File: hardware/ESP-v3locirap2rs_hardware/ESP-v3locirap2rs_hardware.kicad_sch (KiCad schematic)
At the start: 2 parts, among them U1 ESP32-DEVKITC-32D

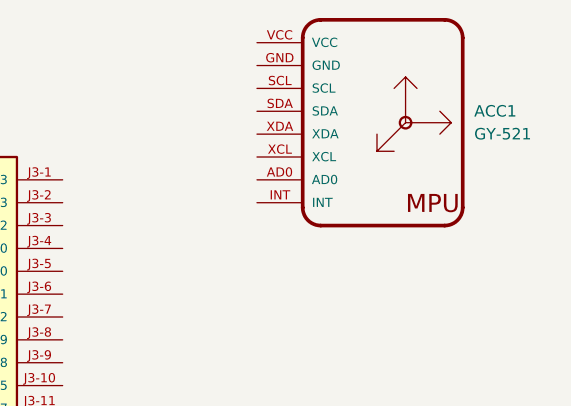
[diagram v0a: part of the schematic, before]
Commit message: updates
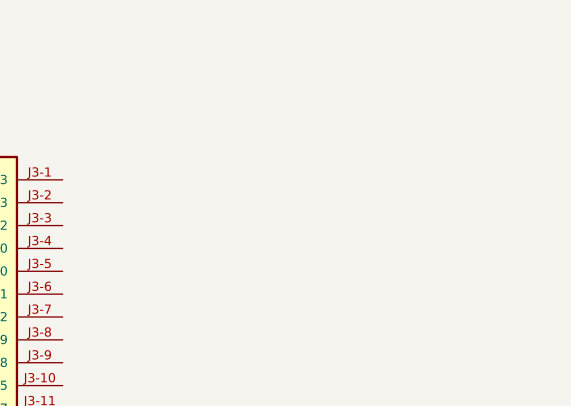
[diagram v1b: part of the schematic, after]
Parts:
- removed ACC1: GY-521, ESP-v3locirap2rs_footprints:GY-521, symbol GY-521:GY-521
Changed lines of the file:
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@@
 	(paper "A4")
-	(symbol
-		(lib_id "GY-521:GY-521")
-		(at 199.39 74.93 0)
-		(unit 1)
-		(exclude_from_sim no)
-		(in_bom yes)
-		(on_board yes)
-		(dnp no)
-		(fields_autoplaced yes)
-		(property "Reference" "ACC1"
-			(at 207.01 73.6599 0)
-			(effects
-				(font
-					(size 1.27 1.27)
-				)
-				(justify left)
-			)
-		)
-		(property "Value" "GY-521"
-			(at 207.01 76.1999 0)
-			(effects
-				(font
-					(size 1.27 1.27)
-				)
-				(justify left)
-			)
-		)
-		(property "Footprint" "ESP-v3locirap2rs_footprints:GY-521"
-			(at 199.39 74.93 0)
-			(effects
-				(font
-					(size 1.27 1.27)
-				)
-				(hide yes)
-			)
-		)
-		(property "Datasheet" ""
-			(at 199.39 74.93 0)
-			(effects
-				(font
-					(size 1.27 1.27)
-				)
-				(hide yes)
-			)
-		)
-		(property "Description" ""
-			(at 199.39 74.93 0)
-			(effects
-				(font
-					(size 1.27 1.27)
-				)
-				(hide yes)
-			)
-		)
-		(property "MF" "GODREAM FORDREAM CO., LIMITED"
-			(at 199.39 74.93 0)
-			(effects
-				(font
-					(size 1.27 1.27)
-				)
-				(justify bottom)
-				(hide yes)
-			)
-		)
-		(property "Description_1" "\n                        \n                            Triple Axis Accelerometer Gyro Breakout\n                        \n"
-			(at 199.39 74.93 0)
-			(effects
-				(font
-					(size 1.27 1.27)
-				)
-				(justify bottom)
-				(hide yes)
-			)
-		)
-		(property "Package" "Package"
-			(at 199.39 74.93 0)
-			(effects
-				(font
-					(size 1.27 1.27)
-				)
-				(justify bottom)
-				(hide yes)
-			)
-		)
-		(property "Price" "None"
-			(at 199.39 74.93 0)
-			(effects
-				(font
-					(size 1.27 1.27)
-				)
-				(justify bottom)
-				(hide yes)
-			)
-		)
-		(property "SnapEDA_Link" "https://www.snapeda.com/parts/GY-521/GODREAM+FORDREAM+CO.%252C+LIMITED/view-part/?ref=snap"
-			(at 199.39 74.93 0)
-			(effects
-				(font
-					(size 1.27 1.27)
-				)
-				(justify bottom)
-				(hide yes)
-			)
-		)
-		(property "MP" "GY-521"
-			(at 199.39 74.93 0)
-			(effects
-				(font
-					(size 1.27 1.27)
-				)
-				(justify bottom)
-				(hide yes)
-			)
-		)
-		(property "Availability" "Not in stock"
-			(at 199.39 74.93 0)
-			(effects
-				(font
-					(size 1.27 1.27)
-				)
-				(justify bottom)
-				(hide yes)
-			)
-		)
-		(property "Check_prices" "https://www.snapeda.com/parts/GY-521/GODREAM+FORDREAM+CO.%252C+LIMITED/view-part/?ref=eda"
-			(at 199.39 74.93 0)
-			(effects
-				(font
-					(size 1.27 1.27)
-				)
-				(justify bottom)
-				(hide yes)
-			)
-		)
-		(pin "VCC"
-		)
-		(pin "SCL"
-		)
-		(pin "XCL"
-		)
-		(pin "AD0"
-		)
-		(pin "SDA"
-		)
-		(pin "XDA"
-		)
-		(pin "GND"
-		)
-		(pin "INT"
-		)
-		(instances
-			(project ""
-				(path "/1e8ac7e4-9b26-4abc-8f5a-d72e2e725c2d"
-					(reference "ACC1")
-					(unit 1)
-				)
-			)
-		)
-	)
 	(symbol
 		(lib_id "ESP32-DEVKITC-32D:ESP32-DEVKITC-32D")

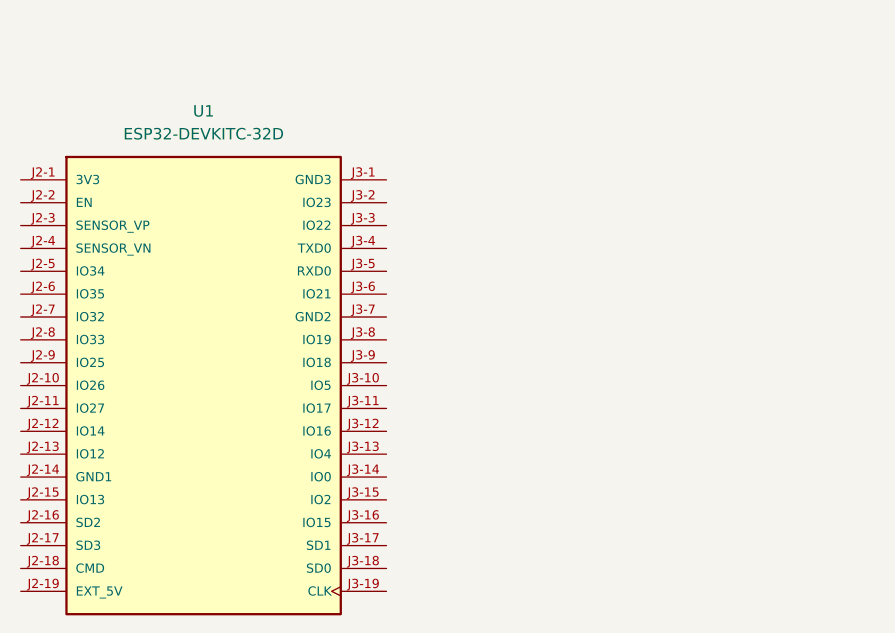
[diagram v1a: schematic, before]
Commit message: circuit diagrams
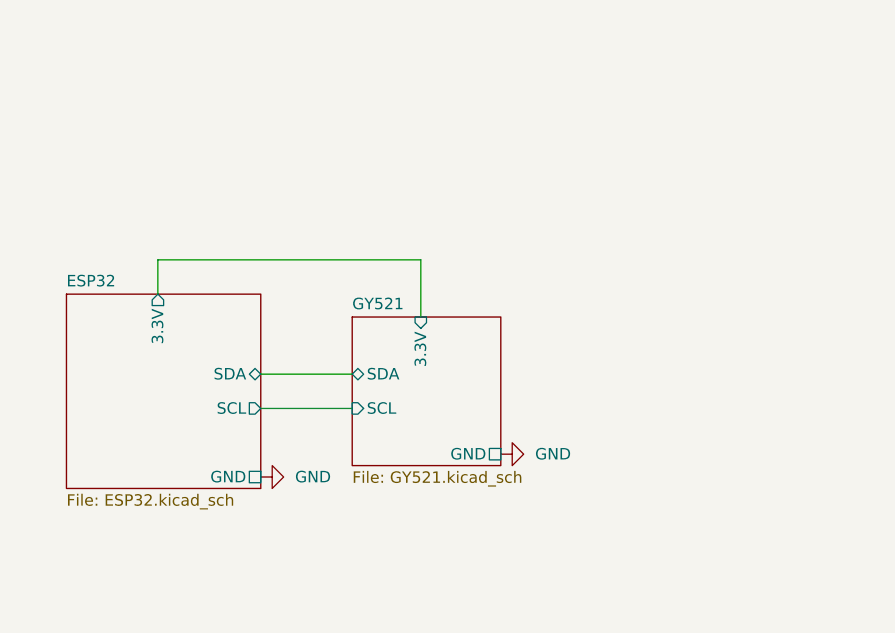
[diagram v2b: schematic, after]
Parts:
- removed U1: ESP32-DEVKITC-32D, digikey-footprints:MODULE_ESP32-DEVKITC-32D, symbol ESP32-DEVKITC-32D:ESP32-DEVKITC-32D
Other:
- added sheet ESP32 (ESP32.kicad_sch)
- added sheet GY521 (GY521.kicad_sch)
